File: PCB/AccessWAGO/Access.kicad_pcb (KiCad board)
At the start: 2 copper layers, 70 x 70 mm, 83 parts, among them J1 USB-C, J10 Reset, J2 NFC, J3 I/O, J4 TC2030-USB-NL-DS, J5 NFC, J6 GND, J7 12V, J8 DOOR, J9 I/O, Q2 PMF250XNEX, SW1 ESE13V01A, U1 MD8942, U10 ESP32-S3-MINI-1, U2 MD8942, U8 G3VM-41GR8

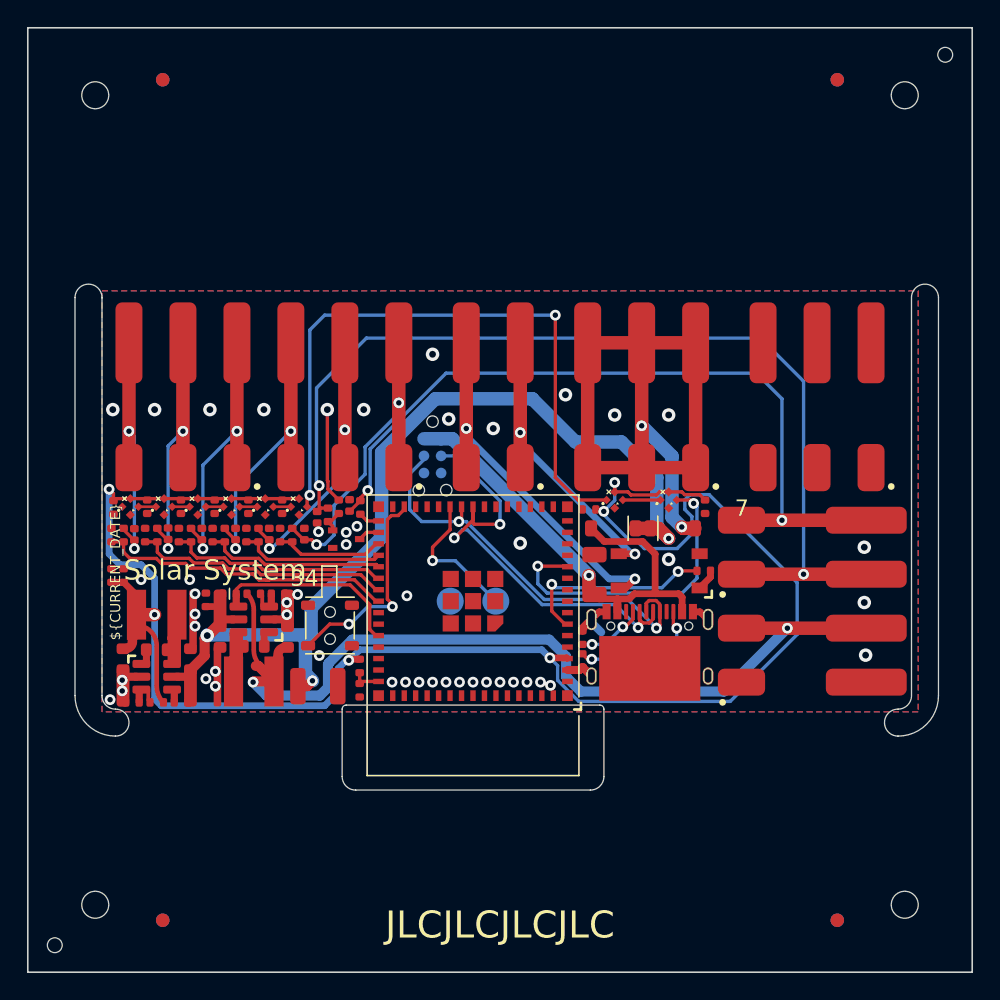
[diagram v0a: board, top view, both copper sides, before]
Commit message: Tidy
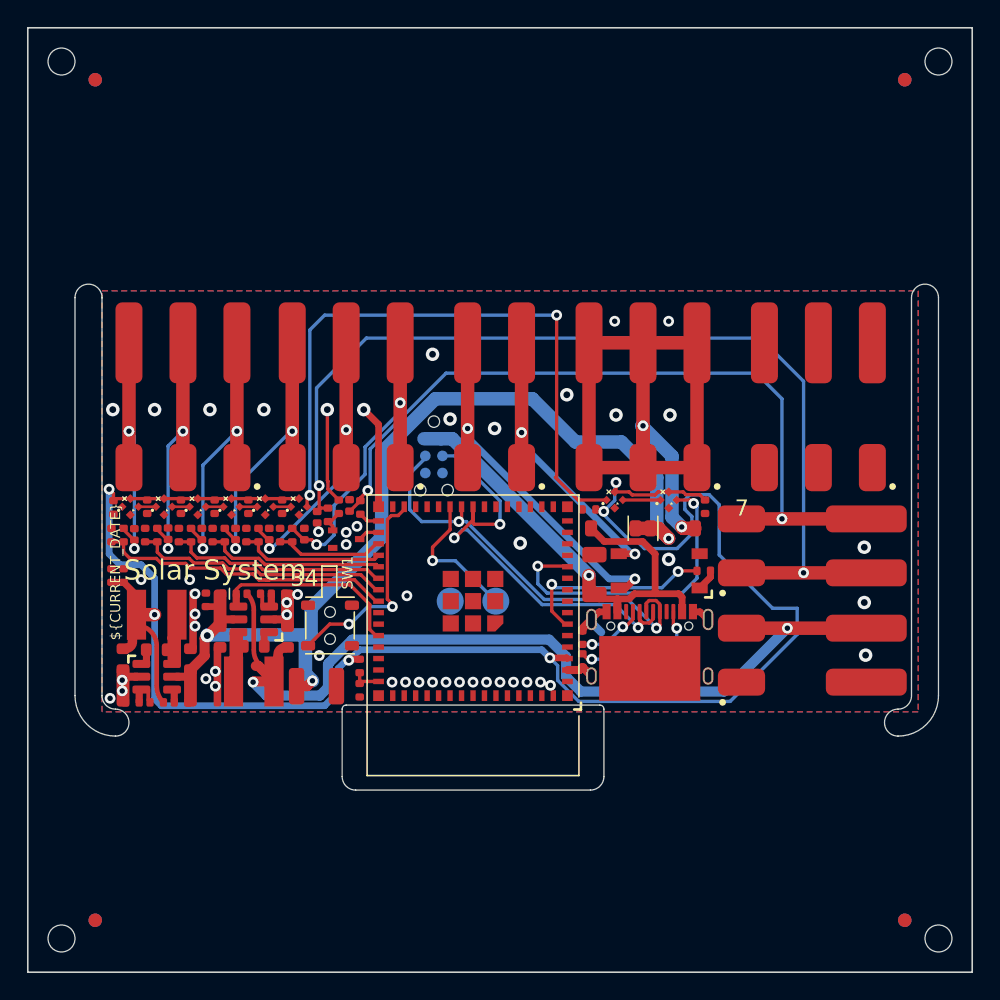
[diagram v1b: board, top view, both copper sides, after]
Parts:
- moved C28 0.10 mm to (88.4, 106.3)
- moved J2 0.10 mm to (124.5, 95.9)
- moved J3 0.10 mm to (90.6, 85.5)
- moved J4 0.10 mm to (97.1, 89.2)
- moved J6 0.10 mm to (125.6, 85.5)
- moved J7 0.10 mm to (112.6, 85.5)
- moved J8 0.10 mm to (101.6, 85.5)
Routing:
- net GND: track 14.3 -> 21.9 mm, vias 50 -> 52
- net +3.3V: track 130.2 -> 131.2 mm
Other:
- board text removed: "15"
- board text removed: "16"
- board text removed: "17"
- board text removed: "18"
- board text removed: "19"
- board text removed: "22"
- board text removed: "23"
